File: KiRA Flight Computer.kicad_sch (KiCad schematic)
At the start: 44 parts, among them J1 Conn_01x04_Pin, J2 USB_C_Receptacle_USB2.0_14P, SW1 SW_Push, SW2 SW_SPDT, U1 ICM-426788P, U2 STM32F407VGTx, U3 MMC5883MA, U4 DPS368, U6 Wio-SX1262, U7 USBLC6-2P6, Y1 16MHz 7pF, Y2 OV_7604

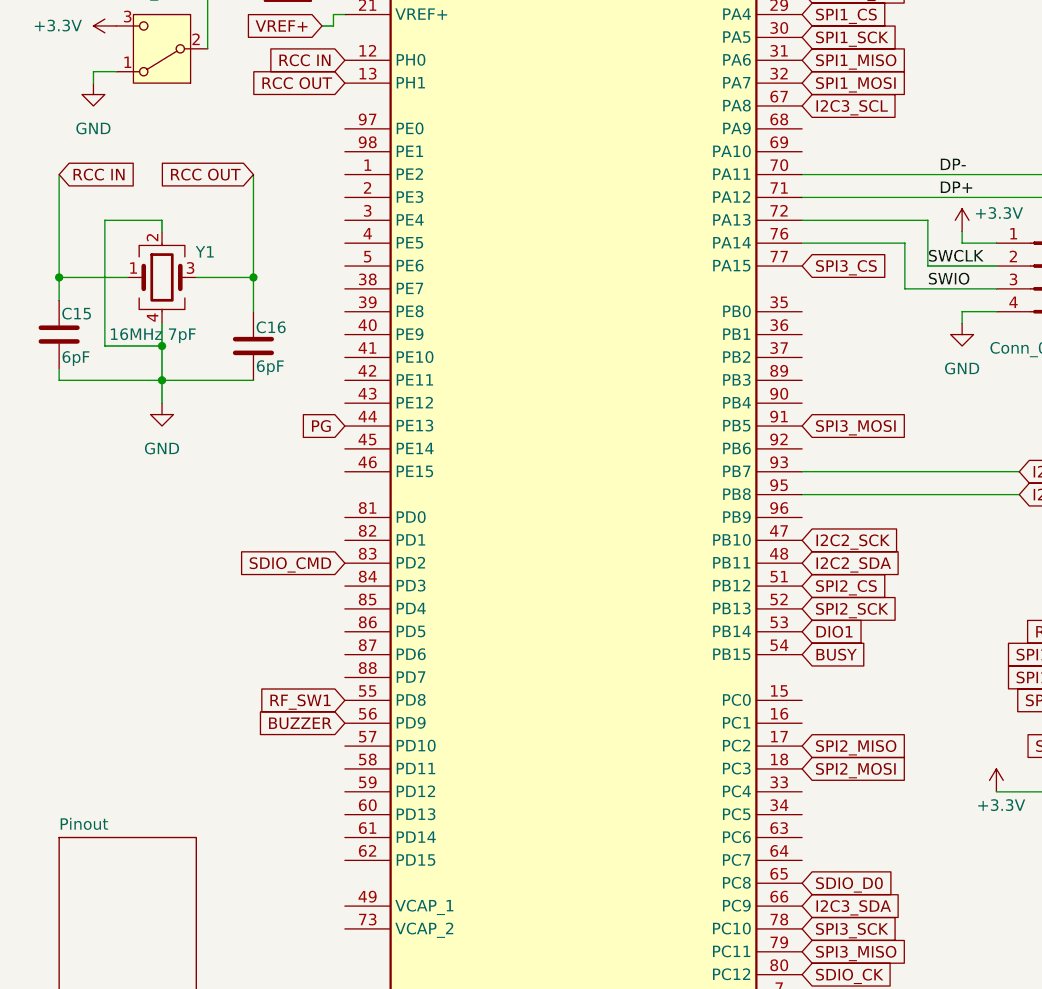
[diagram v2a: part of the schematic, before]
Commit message: Update PCB
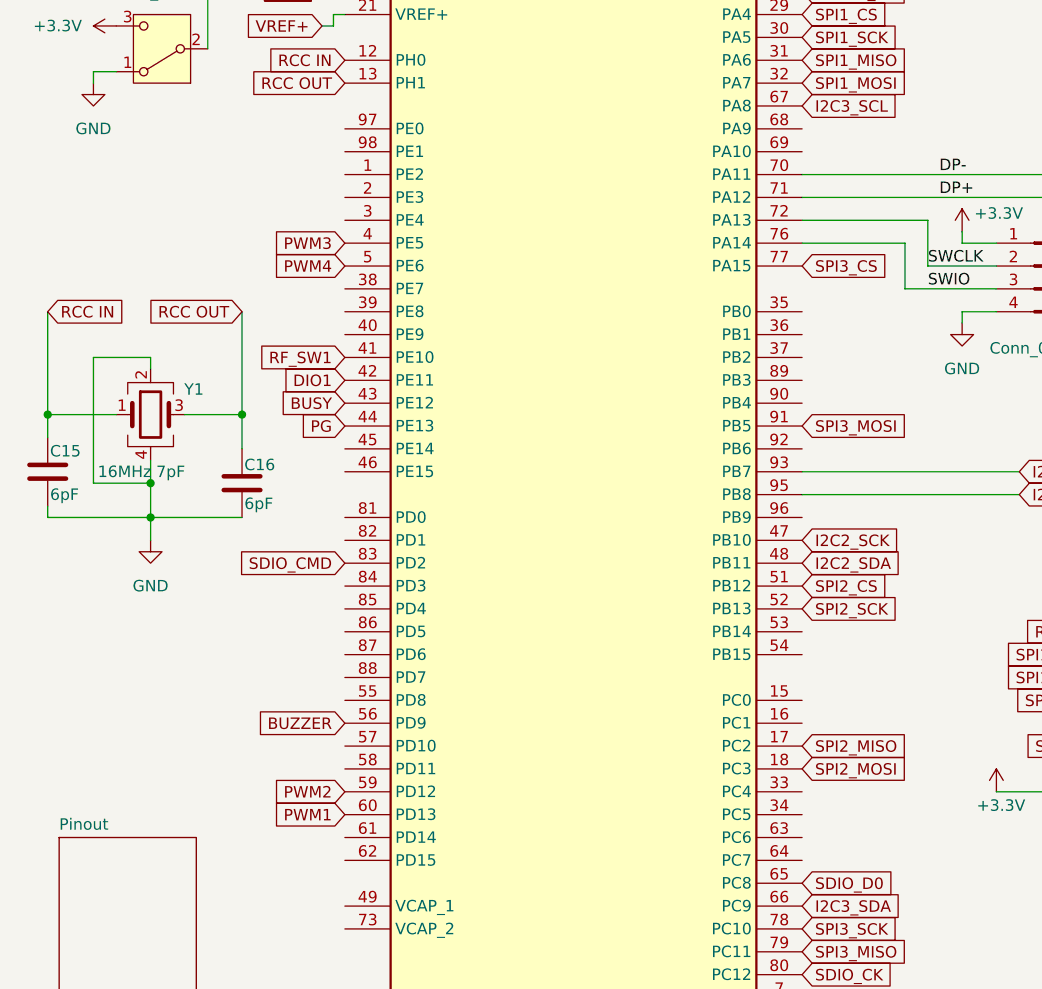
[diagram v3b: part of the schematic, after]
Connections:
- net BUSY: now also U2.43 (PE12); no longer U2.54 (PB15)
- net DIO1: now also U2.42 (PE11); no longer U2.53 (PB14)
- net RF_SW1: now also U2.41 (PE10); no longer U2.55 (PD8)
- net PWM3: now reaches U2.4 (PE5)
- net PWM4: now reaches U2.5 (PE6)
- net PWM2: now reaches U2.59 (PD12)
- net PWM1: now reaches U2.60 (PD13)
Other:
- moved on the sheet: C15, C16, Y1

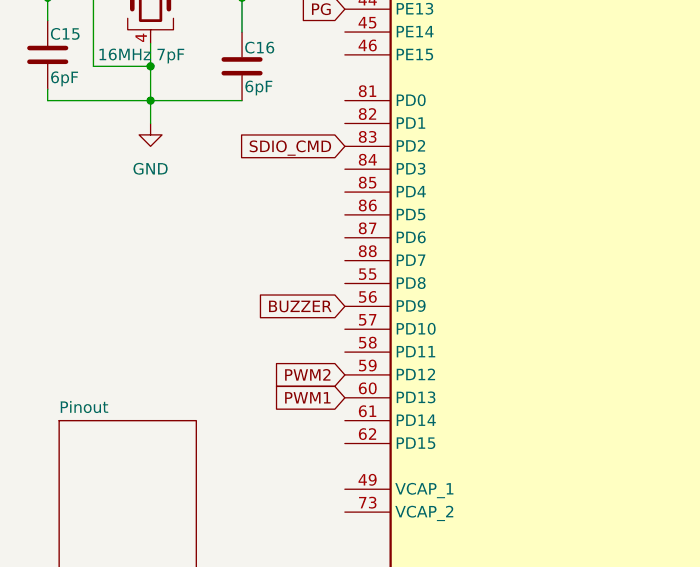
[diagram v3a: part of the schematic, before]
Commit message: questionable changes
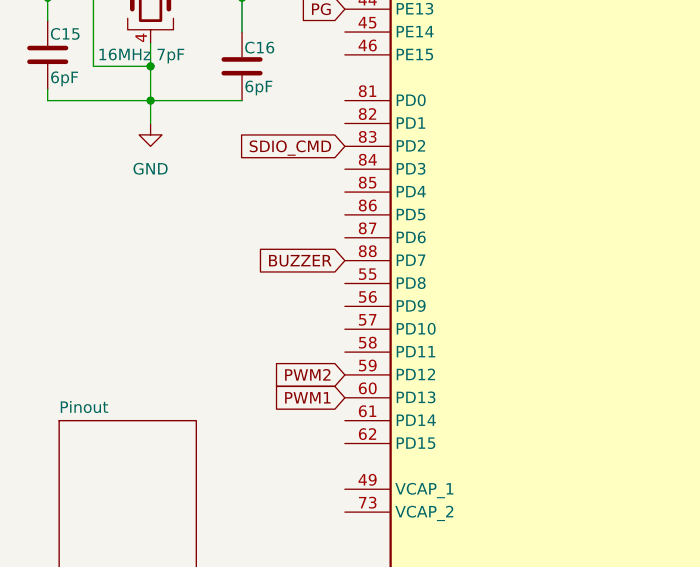
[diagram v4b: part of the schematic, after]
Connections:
- net BUZZER: now also U2.88 (PD7); no longer U2.56 (PD9)
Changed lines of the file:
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@@
 	(global_label "BUZZER"
 		(shape input)
-		(at 48.26 127 180)
+		(at 48.26 121.92 180)
 		(fields_autoplaced yes)
 		(effects
@@
 		)
 		(property "Intersheetrefs" "${INTERSHEET_REFS}"
-			(at 37.8363 127 0)
+			(at 37.8363 121.92 0)
 			(effects
 				(font

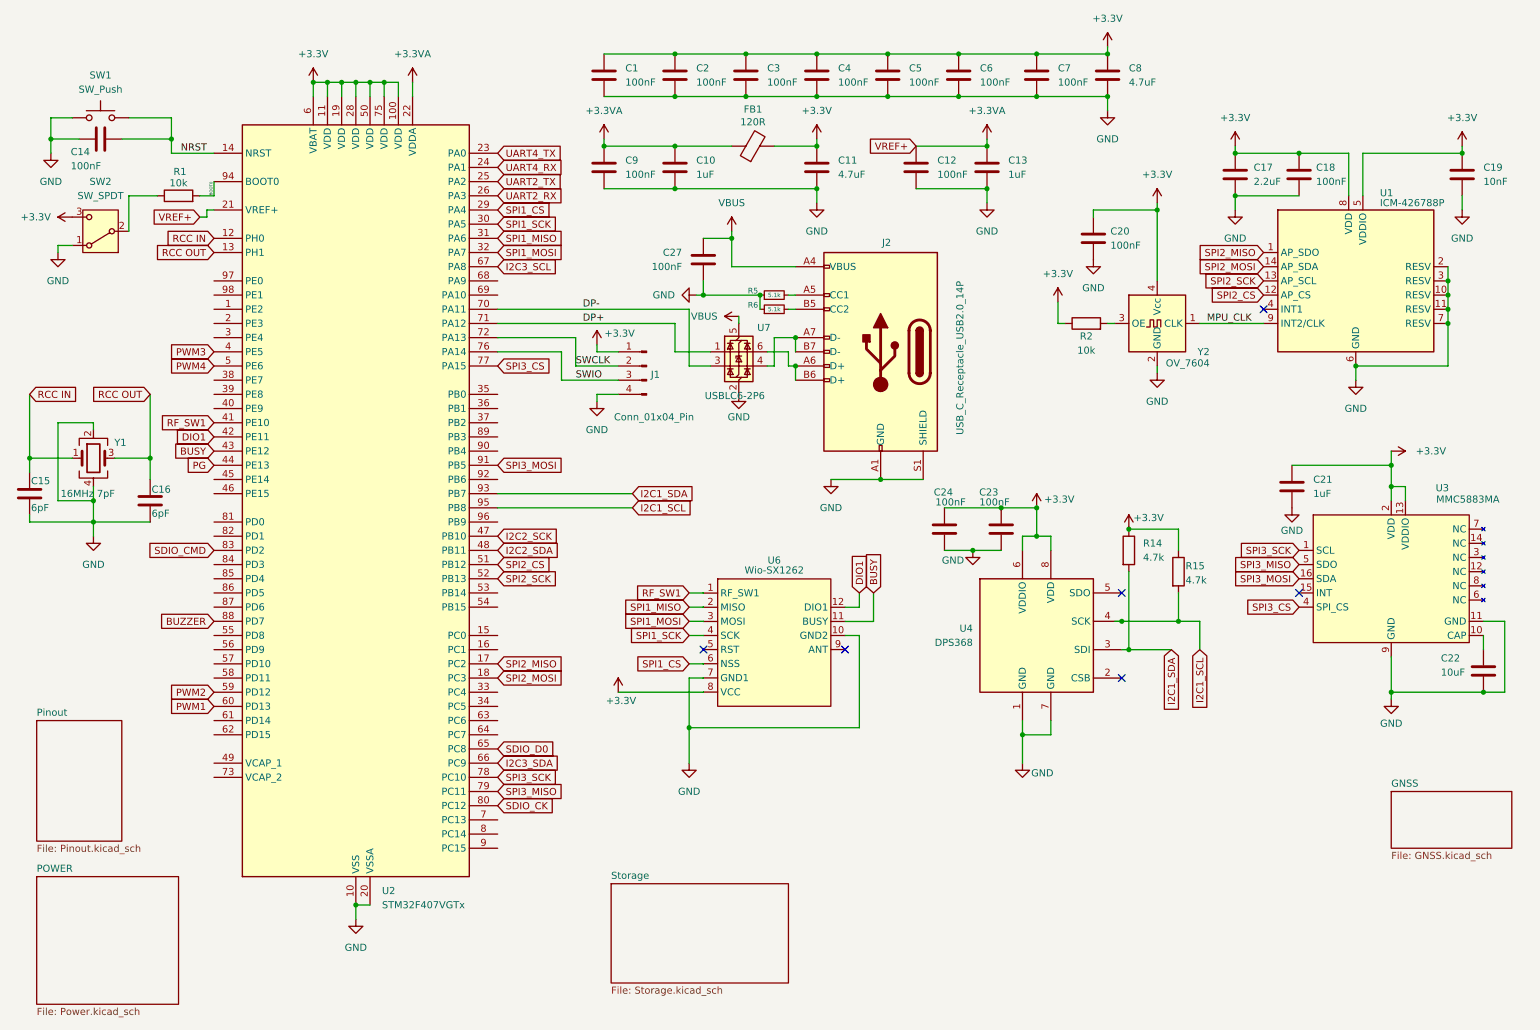
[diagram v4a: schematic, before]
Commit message: PCB Update
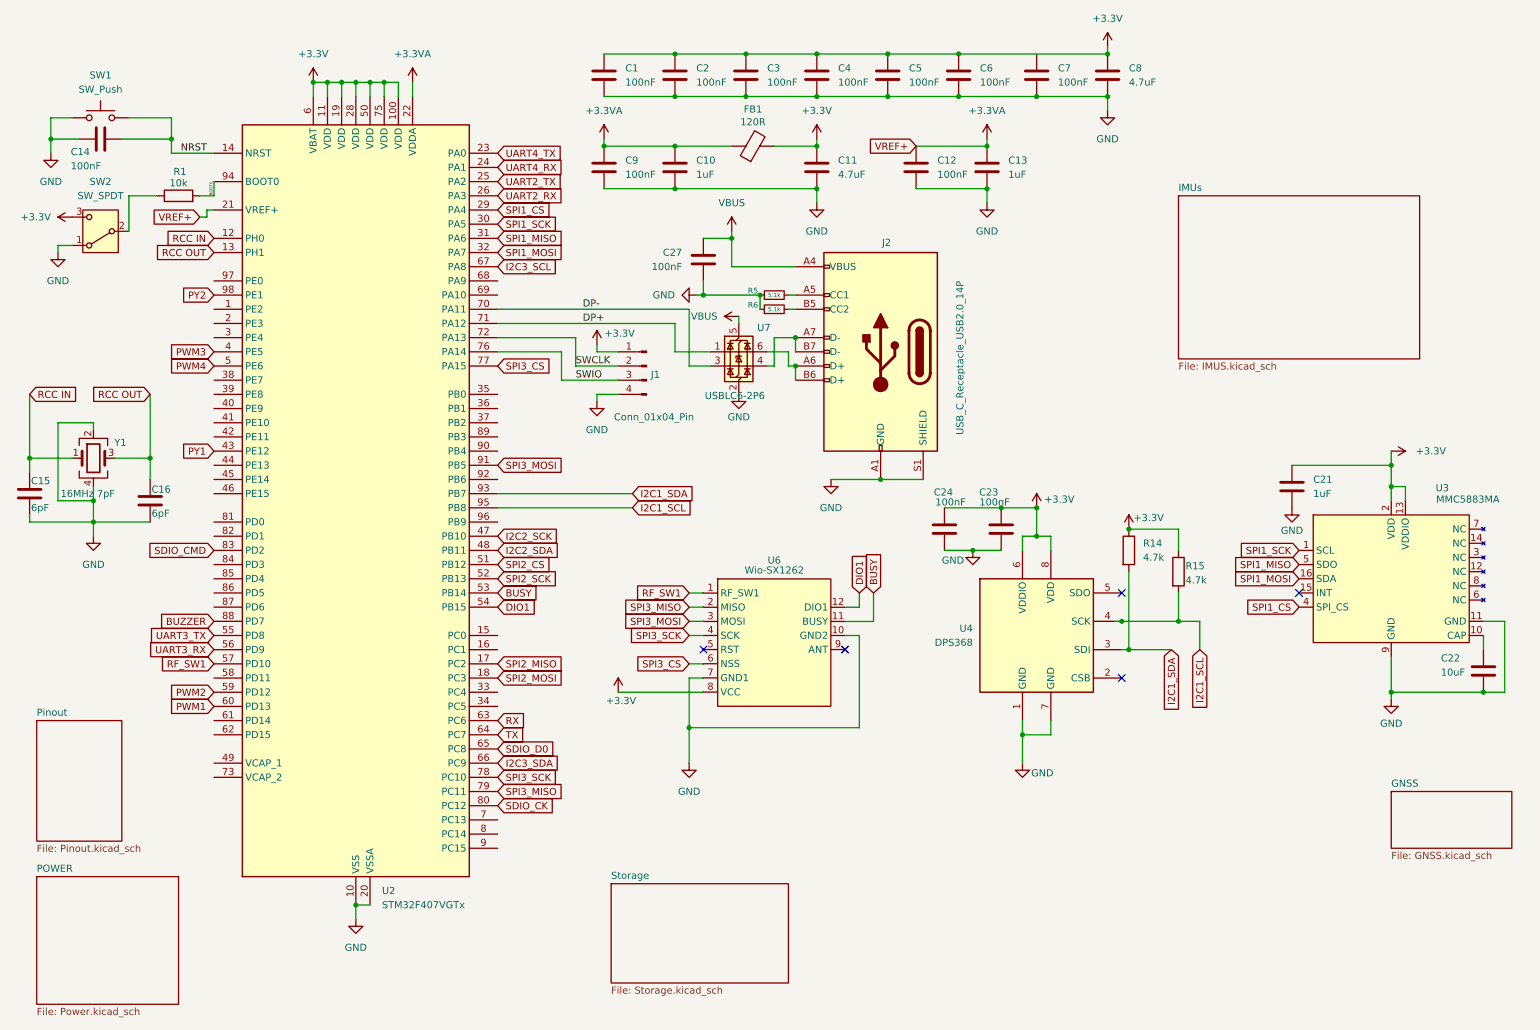
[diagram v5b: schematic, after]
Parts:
- removed C17: 2.2uF, Capacitor_SMD:C_0603_1608Metric, symbol Device:C
- removed C18, C20: 100nF, Capacitor_SMD:C_0603_1608Metric, symbol Device:C
- removed C19: 10nF, Capacitor_SMD:C_0603_1608Metric, symbol Device:C
- removed R2: 10k, Resistor_SMD:R_0603_1608Metric, symbol Device:R
- removed U1: ICM-426788P, Package_LGA:Bosch_LGA-14_3x2.5mm_P0.5mm, symbol Sensor_Motion:BMI160
- removed Y2: OV_7604, Oscillator:Oscillator_SMD_SeikoEpson_SG3030CM, symbol Oscillator:SG-3030CM
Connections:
- net +3.3V: no longer C7.1
- net BUSY: now also U2.53 (PB14); no longer U2.43 (PE12)
- net DIO1: now also U2.54 (PB15); no longer U2.42 (PE11)
- net RF_SW1: now also U2.57 (PD10); no longer U2.41 (PE10)
- net SPI1_CS: now also U3.4 (SPI_CS); no longer U6.6 (NSS)
- net SPI1_MISO: now also U3.5 (SDO); no longer U6.2 (MISO)
- net SPI1_MOSI: now also U3.16 (SDA); no longer U6.3 (MOSI)
- net SPI1_SCK: now also U3.1 (SCL); no longer U6.4 (SCK)
- net SPI3_CS: now also U6.6 (NSS); no longer U3.4 (SPI_CS)
- net SPI3_MISO: now also U6.2 (MISO); no longer U3.5 (SDO)
- net SPI3_MOSI: now also U6.3 (MOSI); no longer U3.16 (SDA)
- net SPI3_SCK: now also U6.4 (SCK); no longer U3.1 (SCL)
- net UART3_TX: now reaches U2.55 (PD8)
- net UART3_RX: now reaches U2.56 (PD9)
- net RX: now reaches U2.63 (PC6)
- net TX: now reaches U2.64 (PC7)
- net PY2: now reaches U2.98 (PE1)
- net PG: no longer names the net of U2.44 (PE13)
- new net PY1: U2.43 (PE12)
- no-connect marks 6 -> 5
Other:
- added sheet IMUs (IMUS.kicad_sch)
